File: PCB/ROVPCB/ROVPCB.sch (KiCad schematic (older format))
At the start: 24 parts, among them J1 Conn_01x04_Male, J2 Conn_01x04_Male, J3 Conn_01x02_Male, J4 Conn_01x01_Male, P1 Conn_02x20_Odd_Even, U1 MPU-9250, U2 BME280, U3 LIGHT_TSL2591, U4 LTC4316IDDPBF, U5 AtlasOEM, U6 LTC2451CTS8-TRMPBF

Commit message: I think it is done!
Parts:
- U4: footprint LTC4316IDDPBF:DFN-10_DD -> Package_SO:MSOP-10_3x3mm_P0.5mm
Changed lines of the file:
@@
 F 0 "U4" H 11525 6015 50  0000 C CNN
 F 1 "LTC4316IDDPBF" H 11525 5924 50  0000 C CNN
-F 2 "LTC4316IDDPBF:DFN-10_DD" H 13450 5150 50  0001 L BNN
+F 2 "Package_SO:MSOP-10_3x3mm_P0.5mm" H 13450 5150 50  0001 L BNN
 F 3 "${KIPRJMOD}\\Datasheets\\LTC4316.pdf" H 13250 5650 50  0001 L BNN
 F 4 "Linear Technology/Analog" H 13100 5950 50  0001 L BNN "Field4"

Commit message: Nothing added just generating Gerbs
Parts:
- MK1, MK2, MK3, MK4: symbol ROVPCB-rescue:Mounting_Hole-Mechanical-ROVPCB-rescue-ROVPCB-rescue -> ROVPCB-rescue:Mounting_Hole-Mechanical-ROVPCB-rescue-ROVPCB-rescue-ROVPCB-rescue
- P1: symbol ROVPCB-rescue:Conn_02x20_Odd_Even-Connector_Generic-ROVPCB-rescue-ROVPCB-rescue -> ROVPCB-rescue:Conn_02x20_Odd_Even-Connector_Generic-ROVPCB-rescue-ROVPCB-rescue-ROVPCB-rescue
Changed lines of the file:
@@
 EESchema Schematic File Version 4
 LIBS:ROVPCB-cache
-EELAYER 26 0
+EELAYER 29 0
 EELAYER END
 $Descr A4 11693 8268
@@
 $EndDescr
 $Comp
-L ROVPCB-rescue:+5V-power-ROVPCB-rescue-ROVPCB-rescue #PWR01
+L ROVPCB-rescue:+5V-power-ROVPCB-rescue-ROVPCB-rescue-ROVPCB-rescue #PWR01
 U 1 1 580C1B61
 P 3100 950
@@
 Connection ~ 3100 1100
 $Comp
-L ROVPCB-rescue:GND-power-ROVPCB-rescue-ROVPCB-rescue #PWR02
+L ROVPCB-rescue:GND-power-ROVPCB-rescue-ROVPCB-rescue-ROVPCB-rescue #PWR02
 U 1 1 580C1D11
 P 3000 3150
@@
 Connection ~ 3000 2000
 $Comp
-L ROVPCB-rescue:GND-power-ROVPCB-rescue-ROVPCB-rescue #PWR03
+L ROVPCB-rescue:GND-power-ROVPCB-rescue-ROVPCB-rescue-ROVPCB-rescue #PWR03
 U 1 1 580C1E01
 P 2300 3150
@@
 	2200 950  2200 1100
 $Comp
-L ROVPCB-rescue:+3.3V-power-ROVPCB-rescue-ROVPCB-rescue #PWR04
+L ROVPCB-rescue:+3.3V-power-ROVPCB-rescue-ROVPCB-rescue-ROVPCB-rescue #PWR04
 U 1 1 580C1BC1
 P 2200 950
@@
 ID_SD and ID_SC PINS:\nThese pins are reserved for HAT ID EEPROM.\n\nAt boot time this I2C interface will be\ninterrogated to look for an EEPROM\nthat identifes the attached board and\nallows automagic setup of the GPIOs\n(and optionally, Linux drivers).\n\nDO NOT USE these pins for anything other\nthan attaching an I2C ID EEPROM. Leave\nunconnected if ID EEPROM not required.
 $Comp
-L ROVPCB-rescue:Mounting_Hole-Mechanical-ROVPCB-rescue-ROVPCB-rescue MK1
+L ROVPCB-rescue:Mounting_Hole-Mechanical-ROVPCB-rescue-ROVPCB-rescue-ROVPCB-rescue MK1
 U 1 1 5834FB2E
 P 3000 7200
@@
 $EndComp
 $Comp
-L ROVPCB-rescue:Mounting_Hole-Mechanical-ROVPCB-rescue-ROVPCB-rescue MK3
+L ROVPCB-rescue:Mounting_Hole-Mechanical-ROVPCB-rescue-ROVPCB-rescue-ROVPCB-rescue MK3
 U 1 1 5834FBEF
 P 3450 7200
@@
 $EndComp
 $Comp
-L ROVPCB-rescue:Mounting_Hole-Mechanical-ROVPCB-rescue-ROVPCB-rescue MK2
+L ROVPCB-rescue:Mounting_Hole-Mechanical-ROVPCB-rescue-ROVPCB-rescue-ROVPCB-rescue MK2
 U 1 1 5834FC19
 P 3000 7400
@@
 $EndComp
 $Comp
-L ROVPCB-rescue:Mounting_Hole-Mechanical-ROVPCB-rescue-ROVPCB-rescue MK4
+L ROVPCB-rescue:Mounting_Hole-Mechanical-ROVPCB-rescue-ROVPCB-rescue-ROVPCB-rescue MK4
 U 1 1 5834FC4F
 P 3450 7400
@@
 Mounting Holes
 $Comp
-L ROVPCB-rescue:Conn_02x20_Odd_Even-Connector_Generic-ROVPCB-rescue-ROVPCB-rescue P1
+L ROVPCB-rescue:Conn_02x20_Odd_Even-Connector_Generic-ROVPCB-rescue-ROVPCB-rescue-ROVPCB-rescue P1
 U 1 1 59AD464A
 P 2600 2000
@@
 GPIO3(SCL1)
 $Comp
-L ROVPCB-rescue:GND-power-ROVPCB-rescue-ROVPCB-rescue #PWR06
+L ROVPCB-rescue:GND-power-ROVPCB-rescue-ROVPCB-rescue-ROVPCB-rescue #PWR06
 U 1 1 5C61D5CB
 P 6250 2200
@@
 $EndComp
 $Comp
-L ROVPCB-rescue:+3.3V-power-ROVPCB-rescue-ROVPCB-rescue #PWR05
+L ROVPCB-rescue:+3.3V-power-ROVPCB-rescue-ROVPCB-rescue-ROVPCB-rescue #PWR05
 U 1 1 5C61D5E4
 P 6000 1300
@@
 $EndComp
 $Comp
-L ROVPCB-rescue:GND-power-ROVPCB-rescue-ROVPCB-rescue #PWR0102
+L ROVPCB-rescue:GND-power-ROVPCB-rescue-ROVPCB-rescue-ROVPCB-rescue #PWR0102
 U 1 1 5C62556F
 P 3050 4450
@@
 $EndComp
 $Comp
-L ROVPCB-rescue:GND-power-ROVPCB-rescue-ROVPCB-rescue #PWR0103
+L ROVPCB-rescue:GND-power-ROVPCB-rescue-ROVPCB-rescue-ROVPCB-rescue #PWR0103
 U 1 1 5C62558E
 P 3050 6200
@@
 $EndComp
 $Comp
-L ROVPCB-rescue:+3.3V-power-ROVPCB-rescue-ROVPCB-rescue #PWR0105
+L ROVPCB-rescue:+3.3V-power-ROVPCB-rescue-ROVPCB-rescue-ROVPCB-rescue #PWR0105
 U 1 1 5C62A4AF
 P 3050 4050
@@
 	3500 5600 3150 5600
 $Comp
-L ROVPCB-rescue:GND-power-ROVPCB-rescue-ROVPCB-rescue #PWR0101
+L ROVPCB-rescue:GND-power-ROVPCB-rescue-ROVPCB-rescue-ROVPCB-rescue #PWR0101
 U 1 1 5CB6C0D3
 P 3350 5700
@@
 Connection ~ 2350 4100
 $Comp
-L ROVPCB-rescue:GND-power-ROVPCB-rescue-ROVPCB-rescue #PWR0106
+L ROVPCB-rescue:GND-power-ROVPCB-rescue-ROVPCB-rescue-ROVPCB-rescue #PWR0106
 U 1 1 5CB74877
 P 1650 5500
@@
 Temp/Press/Humid
 $Comp
-L ROVPCB-rescue:GND-power-ROVPCB-rescue-ROVPCB-rescue #PWR0107
+L ROVPCB-rescue:GND-power-ROVPCB-rescue-ROVPCB-rescue-ROVPCB-rescue #PWR0107
 U 1 1 5CB8835A
 P 5300 5950
@@
 $EndComp
 $Comp
-L ROVPCB-rescue:GND-power-ROVPCB-rescue-ROVPCB-rescue #PWR0108
+L ROVPCB-rescue:GND-power-ROVPCB-rescue-ROVPCB-rescue-ROVPCB-rescue #PWR0108
 U 1 1 5CB8AB73
 P 4700 4850
@@
 $EndComp
 $Comp
-L ROVPCB-rescue:+3.3V-power-ROVPCB-rescue-ROVPCB-rescue #PWR0109
+L ROVPCB-rescue:+3.3V-power-ROVPCB-rescue-ROVPCB-rescue-ROVPCB-rescue #PWR0109
 U 1 1 5CB8D386
 P 5300 4450
@@
 	5200 4750 5300 4750
 $Comp
-L ROVPCB-rescue:+3.3V-power-ROVPCB-rescue-ROVPCB-rescue #PWR0110
+L ROVPCB-rescue:+3.3V-power-ROVPCB-rescue-ROVPCB-rescue-ROVPCB-rescue #PWR0110
 U 1 1 5CB8FE0A
 P 6050 5650
@@
 $EndComp
 $Comp
-L ROVPCB-rescue:+3.3V-power-ROVPCB-rescue-ROVPCB-rescue #PWR07
+L ROVPCB-rescue:+3.3V-power-ROVPCB-rescue-ROVPCB-rescue-ROVPCB-rescue #PWR07
 U 1 1 5CB72608
 P 4400 7250
@@
 	4400 7250 4750 7250
 $Comp
-L ROVPCB-rescue:GND-power-ROVPCB-rescue-ROVPCB-rescue #PWR08
+L ROVPCB-rescue:GND-power-ROVPCB-rescue-ROVPCB-rescue-ROVPCB-rescue #PWR08
 U 1 1 5CB7546E
 P 4600 7350
@@
 	7000 5250 7500 5250
 $Comp
-L ROVPCB-rescue:GND-power-ROVPCB-rescue-ROVPCB-rescue #PWR0111
+L ROVPCB-rescue:GND-power-ROVPCB-rescue-ROVPCB-rescue-ROVPCB-rescue #PWR0111
 U 1 1 5CB8FA80
 P 7500 6000
@@
 	6750 5450 7500 5450
 $Comp
-L ROVPCB-rescue:GND-power-ROVPCB-rescue-ROVPCB-rescue #PWR0112
+L ROVPCB-rescue:GND-power-ROVPCB-rescue-ROVPCB-rescue-ROVPCB-rescue #PWR0112
 U 1 1 5CBA3506
 P 9250 5550
@@
 	9250 5550 9150 5550
 $Comp
-L ROVPCB-rescue:+3.3V-power-ROVPCB-rescue-ROVPCB-rescue #PWR0113
+L ROVPCB-rescue:+3.3V-power-ROVPCB-rescue-ROVPCB-rescue-ROVPCB-rescue #PWR0113
 U 1 1 5CBA6BEC
 P 9350 5350
@@
 Default I2C address--Temp: 0x77; Pressure: 0x76
 $Comp
-L ROVPCB-rescue:GND-power-ROVPCB-rescue-ROVPCB-rescue #PWR0114
+L ROVPCB-rescue:GND-power-ROVPCB-rescue-ROVPCB-rescue-ROVPCB-rescue #PWR0114
 U 1 1 5CBDF2B2
 P 6200 4900
@@
 	9550 1450 9000 1450
 $Comp
-L ROVPCB-rescue:GND-power-ROVPCB-rescue-ROVPCB-rescue #PWR010
+L ROVPCB-rescue:GND-power-ROVPCB-rescue-ROVPCB-rescue-ROVPCB-rescue #PWR010
 U 1 1 5CBFDF85
 P 9250 1650
@@
 	9250 1650 9000 1650
 $Comp
-L ROVPCB-rescue:+3.3V-power-ROVPCB-rescue-ROVPCB-rescue #PWR09
+L ROVPCB-rescue:+3.3V-power-ROVPCB-rescue-ROVPCB-rescue-ROVPCB-rescue #PWR09
 U 1 1 5CC01F57
 P 7750 1450
@@
 	8300 1750 8100 1750
 $Comp
-L ROVPCB-rescue:GND-power-ROVPCB-rescue-ROVPCB-rescue #PWR011
+L ROVPCB-rescue:GND-power-ROVPCB-rescue-ROVPCB-rescue-ROVPCB-rescue #PWR011
 U 1 1 5CBE8F10
 P 1000 5100
@@
 	10150 2850 9500 2850
 $Comp
-L ROVPCB-rescue:GND-power-ROVPCB-rescue-ROVPCB-rescue #PWR0104
+L ROVPCB-rescue:GND-power-ROVPCB-rescue-ROVPCB-rescue-ROVPCB-rescue #PWR0104
 U 1 1 5CC19AEF
 P 9750 3400
@@
 $EndComp
 $Comp
-L ROVPCB-rescue:GND-power-ROVPCB-rescue-ROVPCB-rescue #PWR0115
+L ROVPCB-rescue:GND-power-ROVPCB-rescue-ROVPCB-rescue-ROVPCB-rescue #PWR0115
 U 1 1 5CC19B4E
 P 7900 2850
@@
 	8150 2850 7900 2850
 $Comp
-L ROVPCB-rescue:+3.3V-power-ROVPCB-rescue-ROVPCB-rescue #PWR0116
+L ROVPCB-rescue:+3.3V-power-ROVPCB-rescue-ROVPCB-rescue-ROVPCB-rescue #PWR0116
 U 1 1 5CC1F2DC
 P 7650 3150
@@
 Connection ~ 8150 3150
 $Comp
-L ROVPCB-rescue:GND-power-ROVPCB-rescue-ROVPCB-rescue #PWR0117
+L ROVPCB-rescue:GND-power-ROVPCB-rescue-ROVPCB-rescue-ROVPCB-rescue #PWR0117
 U 1 1 5CC40D88
 P 8050 3550
@@
 $EndComp
 $Comp
-L ROVPCB-rescue:GND-power-ROVPCB-rescue-ROVPCB-rescue #PWR0118
+L ROVPCB-rescue:GND-power-ROVPCB-rescue-ROVPCB-rescue-ROVPCB-rescue #PWR0118
 U 1 1 5CC46ADC
 P 7650 3550

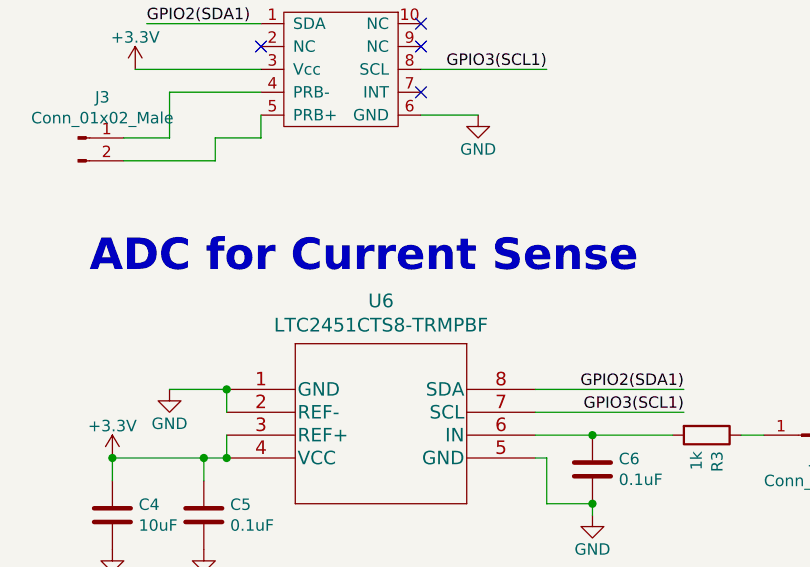
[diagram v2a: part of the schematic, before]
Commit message: Added some documentation stuffs
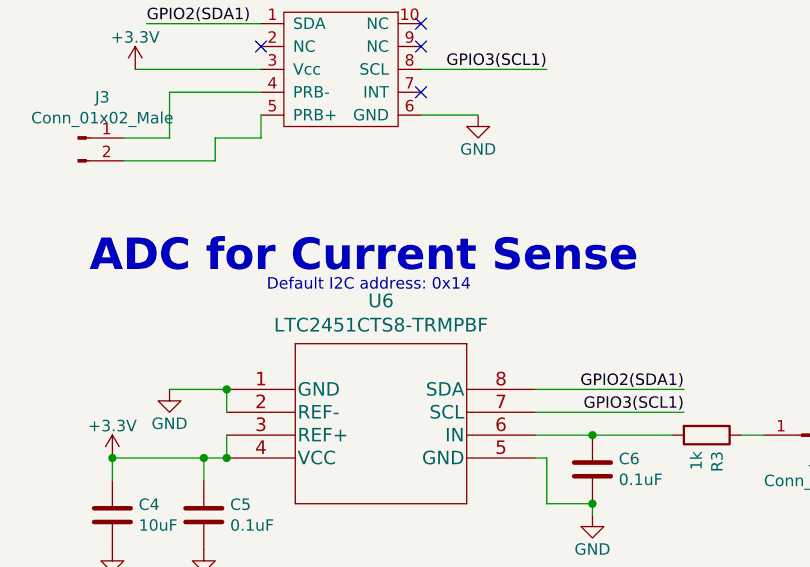
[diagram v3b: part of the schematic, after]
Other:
- note added: "Default I2C address: 0x14"
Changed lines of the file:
@@
 Wire Wire Line
 	2300 3000 2300 3150
+Text Notes 8325 2425 0    50   ~ 0
+Default I2C address: 0x14
 $EndSCHEMATC
